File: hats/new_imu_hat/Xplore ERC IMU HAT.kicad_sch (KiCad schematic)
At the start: 36 parts, among them J1 BM08B-GHS-TBT, J2 5025850570, J3 BM04B-GHS-TBT, J4 Hat_connector_hole, J5 5025850670, SW1 SW_DIP_x01, U1 LT3960JMSE-PBF

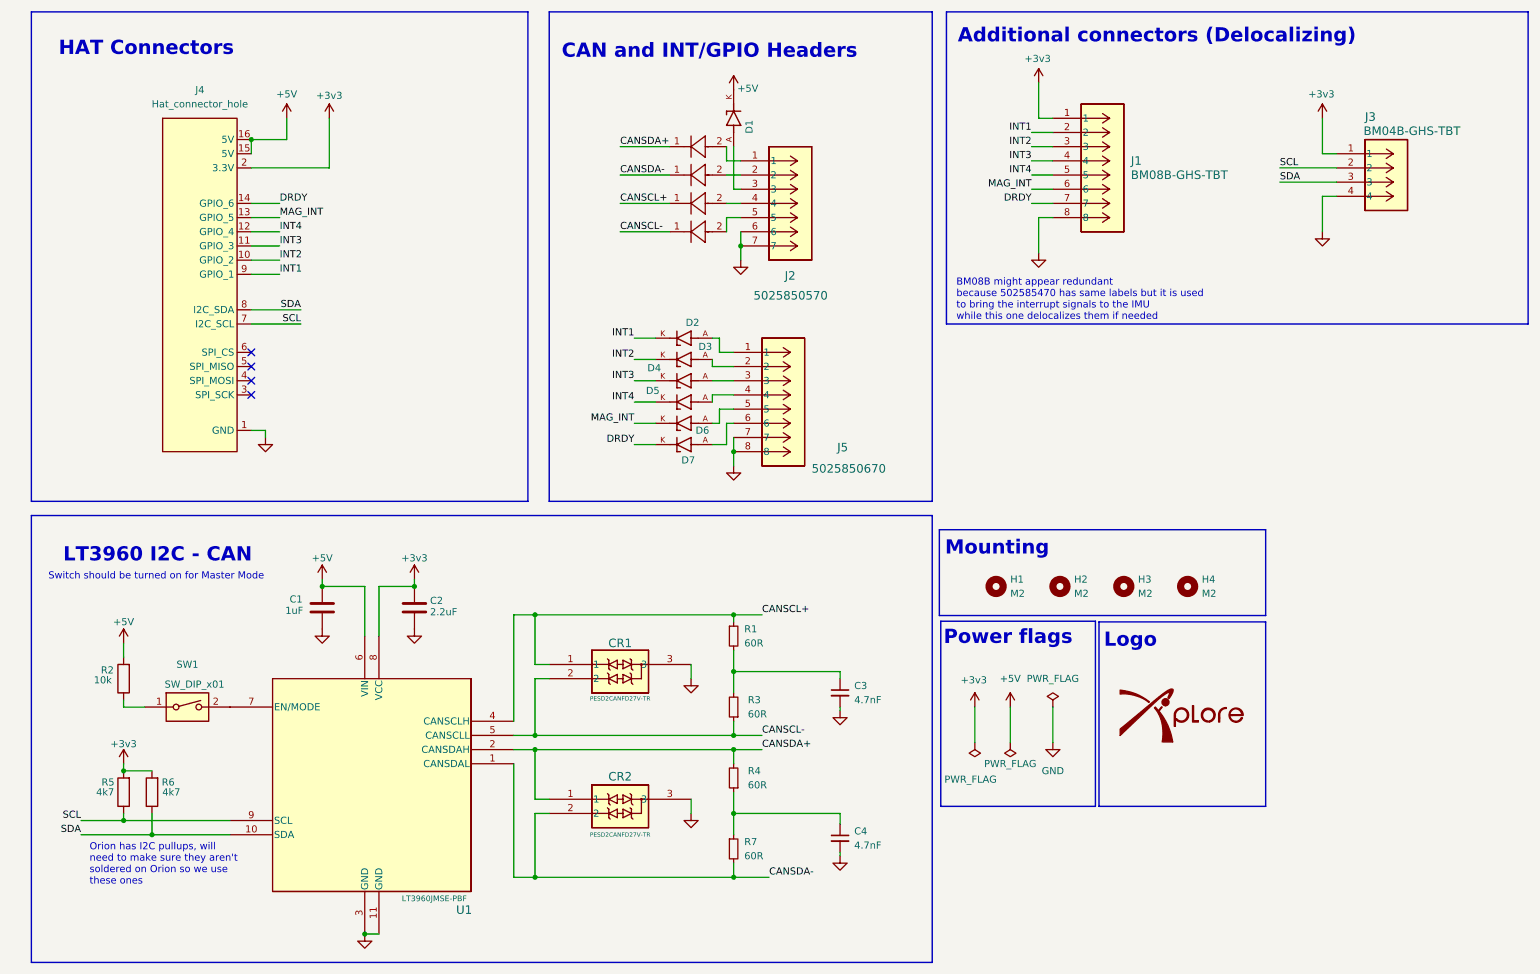
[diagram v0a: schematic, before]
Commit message: IMU v4.1, fixed diode selection
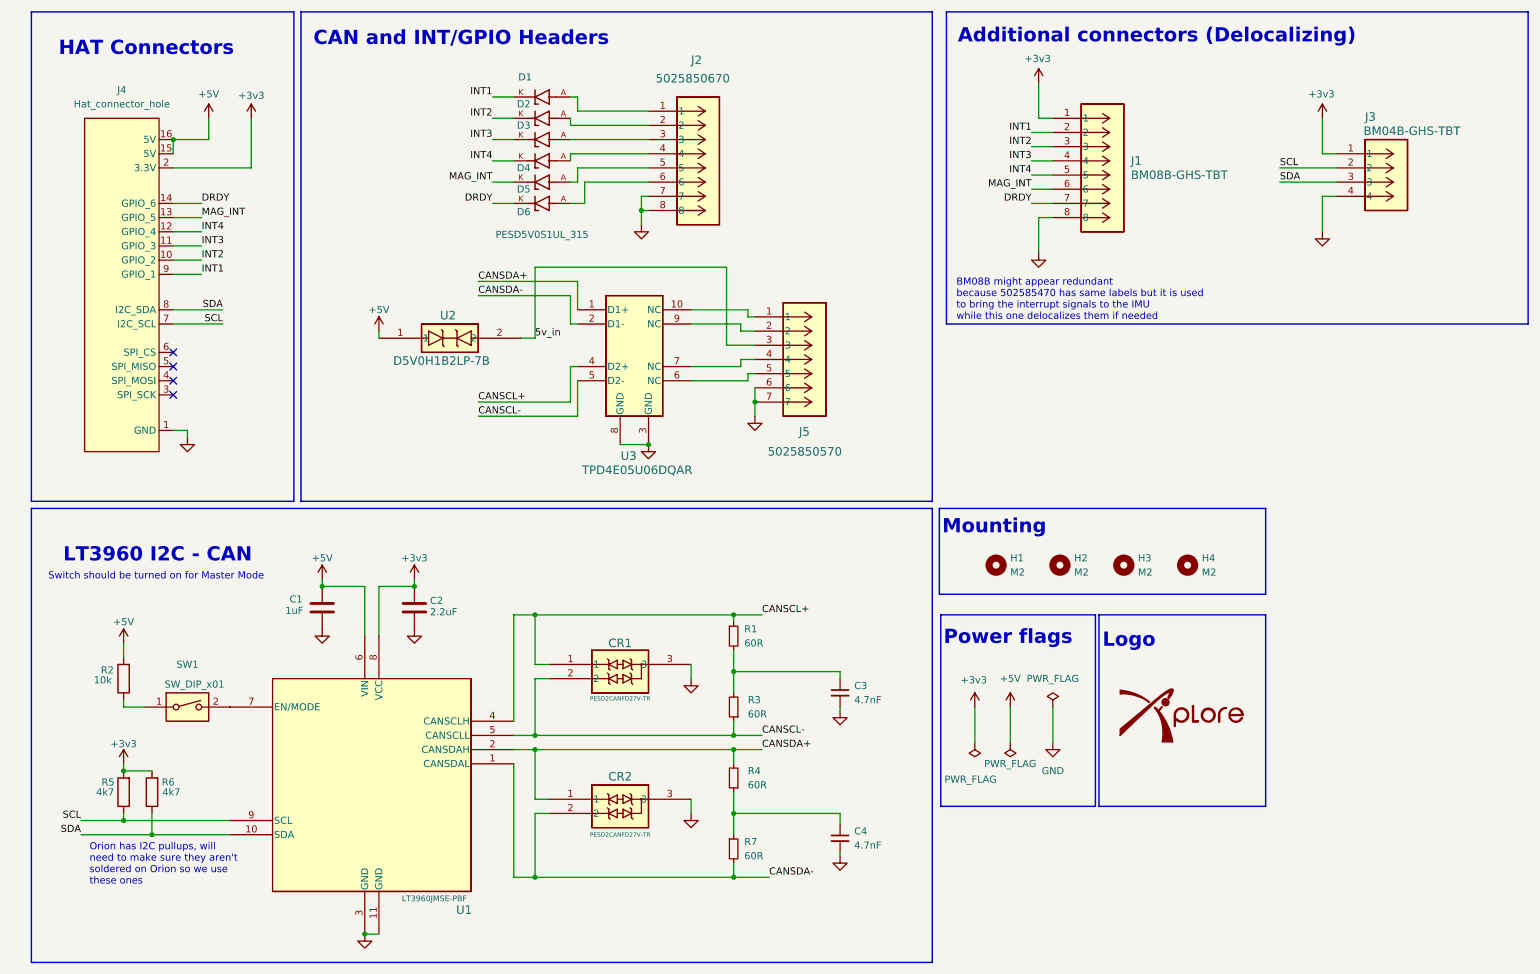
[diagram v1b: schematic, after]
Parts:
- removed CR3, CR4, CR5, CR6: CDSOD323-T05C, footprints:DIODE_CDSOD323-T05C_BRN, symbol CDSOD323_T05C:CDSOD323-T05C
- removed D7: PESD5V0S1UL_315, footprints:DIO_PESD5V0S1UL_315, symbol PESD5V0S1UL_315:PESD5V0S1UL_315
- removed J2: 5025850570, footprints:CON_5025850570, symbol 5025850570:5025850570
- removed J5: 5025850670, footprints:CON_5025850670, symbol 502585670:5025850670
- added J2: 5025850670, footprints:CON_5025850670, symbol 502585670:5025850670
- added J5: 5025850570, footprints:CON_5025850570, symbol 5025850570:5025850570
- added U2: D5V0H1B2LP-7B, footprints:D5V0H1B2LP_7B, symbol D5V0H1B2LP_7B:D5V0H1B2LP-7B
- added U3: TPD4E05U06DQAR, footprints:TPD4E05U06DQAR, symbol TPD4E05U06DQAR:TPD4E05U06DQAR
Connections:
- net +5V: now also U2.1; no longer D1.K
- net CANSCL+: now also U3.4 (D2+)
- net CANSCL-: now also U3.5 (D2-)
- net CANSDA+: now also U3.1 (D1+)
- net CANSDA-: now also U3.2 (D1-)
- net DRDY: now also D6.K
- net GND: now also J2.7, J2.8, J5.6, J5.7, U3.3 (GND), U3.8 (GND)
- net INT1: now also D1.K; no longer D2.K
- net INT2: now also D2.K; no longer D3.K
- net INT3: now also D3.K; no longer D4.K
- net INT4: now also D4.K; no longer D5.K
- net MAG_INT: now also D5.K; no longer D6.K
- net at D4.A: now also J2.4
- net at D5.A: now also J2.5
- net at D3.A: now also J2.3
- net at D2.A: now also J2.2
- net at D6.A: now also J2.6
- net at D1.A: now also J2.1
- new net: J5.1, U3.10 (NC)
- new net: J5.2, U3.9 (NC)
- new net: J5.4, U3.7 (NC)
- new net: J5.5, U3.6 (NC)
- new net 5v_in: J5.3, U2.2
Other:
- moved on the sheet: H1, H2, H3, H4, J4
